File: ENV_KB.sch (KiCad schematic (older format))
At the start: 178 parts, among them P1 USB_C_Plug_USB2.0

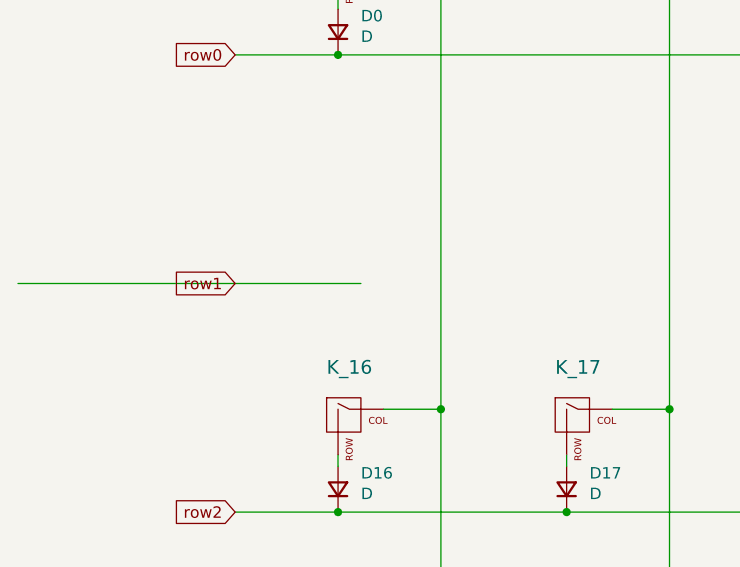
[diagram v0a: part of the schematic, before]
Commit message: some random changes
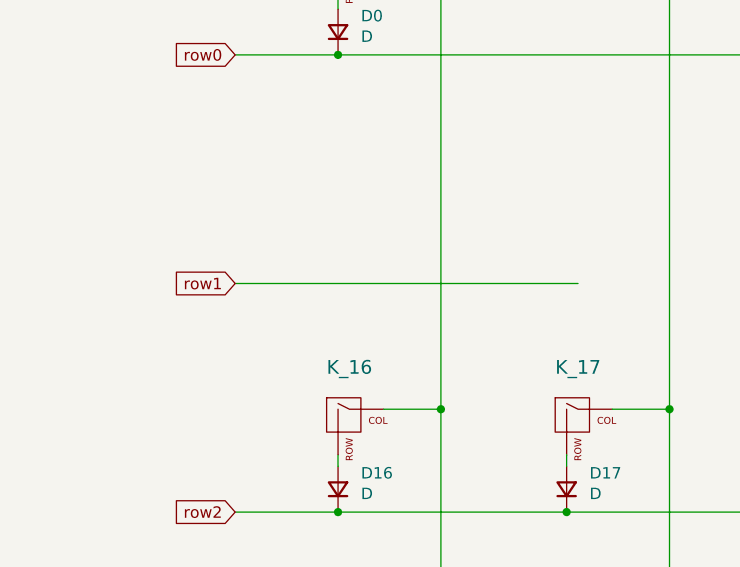
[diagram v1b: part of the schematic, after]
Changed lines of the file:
@@
 	1350 3400 2350 3400
 Wire Wire Line
-	-50  2400 1450 2400
+	900  2400 2400 2400
 Wire Wire Line
 	1350 1400 3350 1400
@@
 $Comp
 L MX_Alps_Hybrid:MX-NoLED K_0
-U 1 1 00000001
+U 1 1 603522C8
 P 1400 1000
 F 0 "K_0" H 1400 1233 60  0000 C CNN
@@
 $Comp
 L MX_Alps_Hybrid:MX-NoLED K_1
-U 1 1 00000011
+U 1 1 603522CA
 P 3400 1000
 F 0 "K_1" H 3400 1233 60  0000 C CNN
@@
 $Comp
 L MX_Alps_Hybrid:MX-NoLED K_3
-U 1 1 00000031
+U 1 1 603522CE
 P 5400 1000
 F 0 "K_3" H 5400 1233 60  0000 C CNN
@@
 $Comp
 L MX_Alps_Hybrid:MX-NoLED K_4
-U 1 1 00000041
+U 1 1 603522D0
 P 6400 1000
 F 0 "K_4" H 6400 1233 60  0000 C CNN
@@
 $Comp
 L MX_Alps_Hybrid:MX-NoLED K_5
-U 1 1 00000051
+U 1 1 603522D2
 P 8400 1000
 F 0 "K_5" H 8400 1233 60  0000 C CNN
@@
 $Comp
 L MX_Alps_Hybrid:MX-NoLED K_7
-U 1 1 00000071
+U 1 1 603522D6
 P 10400 1000
 F 0 "K_7" H 10400 1233 60  0000 C CNN
@@
 $Comp
 L Device:D_Small D7
-U 1 1 00000070
+U 1 1 603522D5
 P 10350 1300
 F 0 "D7" V 10420 1200 50  0000 R CNN
@@
 $Comp
 L Device:D_Small D8
-U 1 1 00000080
+U 1 1 603522D7
 P 11350 1300
 F 0 "D8" V 11420 1200 50  0000 R CNN
@@
 $Comp
 L MX_Alps_Hybrid:MX-NoLED K_9
-U 1 1 00000091
+U 1 1 603522DA
 P 12400 1000
 F 0 "K_9" H 12400 1233 60  0000 C CNN
@@
 $Comp
 L Device:D_Small D9
-U 1 1 00000090
+U 1 1 603522D9
 P 12350 1300
 F 0 "D9" V 12420 1200 50  0000 R CNN
@@
 $Comp
 L MX_Alps_Hybrid:MX-NoLED K_10
-U 1 1 00000101
+U 1 1 603522DC
 P 13400 1000
 F 0 "K_10" H 13400 1233 60  0000 C CNN
@@
 $Comp
 L Device:D_Small D6
-U 1 1 00000060
+U 1 1 603522D3
 P 9350 1300
 F 0 "D6" V 9420 1200 50  0000 R CNN
@@
 $Comp
 L Device:D_Small D5
-U 1 1 00000050
+U 1 1 603522D1
 P 8350 1300
 F 0 "D5" V 8420 1200 50  0000 R CNN
@@
 $Comp
 L Device:D_Small D4
-U 1 1 00000040
+U 1 1 603522CF
 P 6350 1300
 F 0 "D4" V 6420 1200 50  0000 R CNN
@@
 $Comp
 L Device:D_Small D3
-U 1 1 00000030
+U 1 1 603522CD
 P 5350 1300
 F 0 "D3" V 5420 1200 50  0000 R CNN
@@
 $Comp
 L Device:D_Small D2
-U 1 1 00000020
+U 1 1 603522CB
 P 4350 1300
 F 0 "D2" V 4420 1200 50  0000 R CNN
